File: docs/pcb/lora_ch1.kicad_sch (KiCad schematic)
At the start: 22 parts, among them J2 TYPE-C-31-M-12, J3 JST_2mm_LiPo, U1 ESP32-C3_SUPERMINI_TH, U2 TP4056-42-ESOP8, U3 DRV2605LDGS, U4 AP2112K-3.3

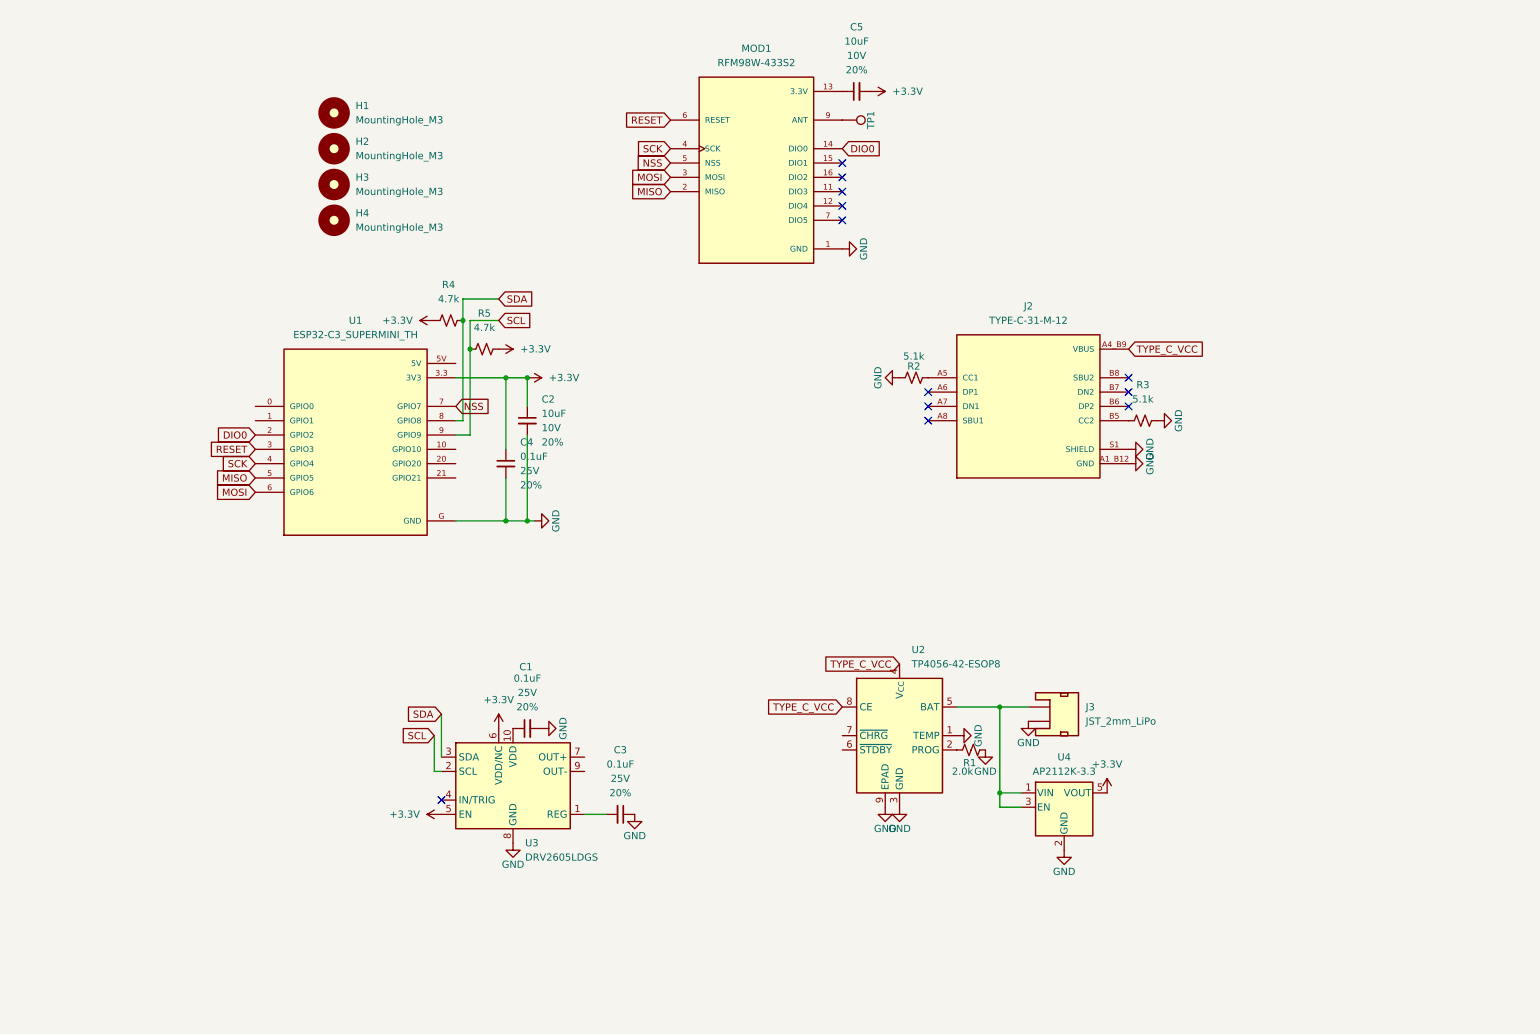
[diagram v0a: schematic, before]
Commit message: PCB schematic finished.
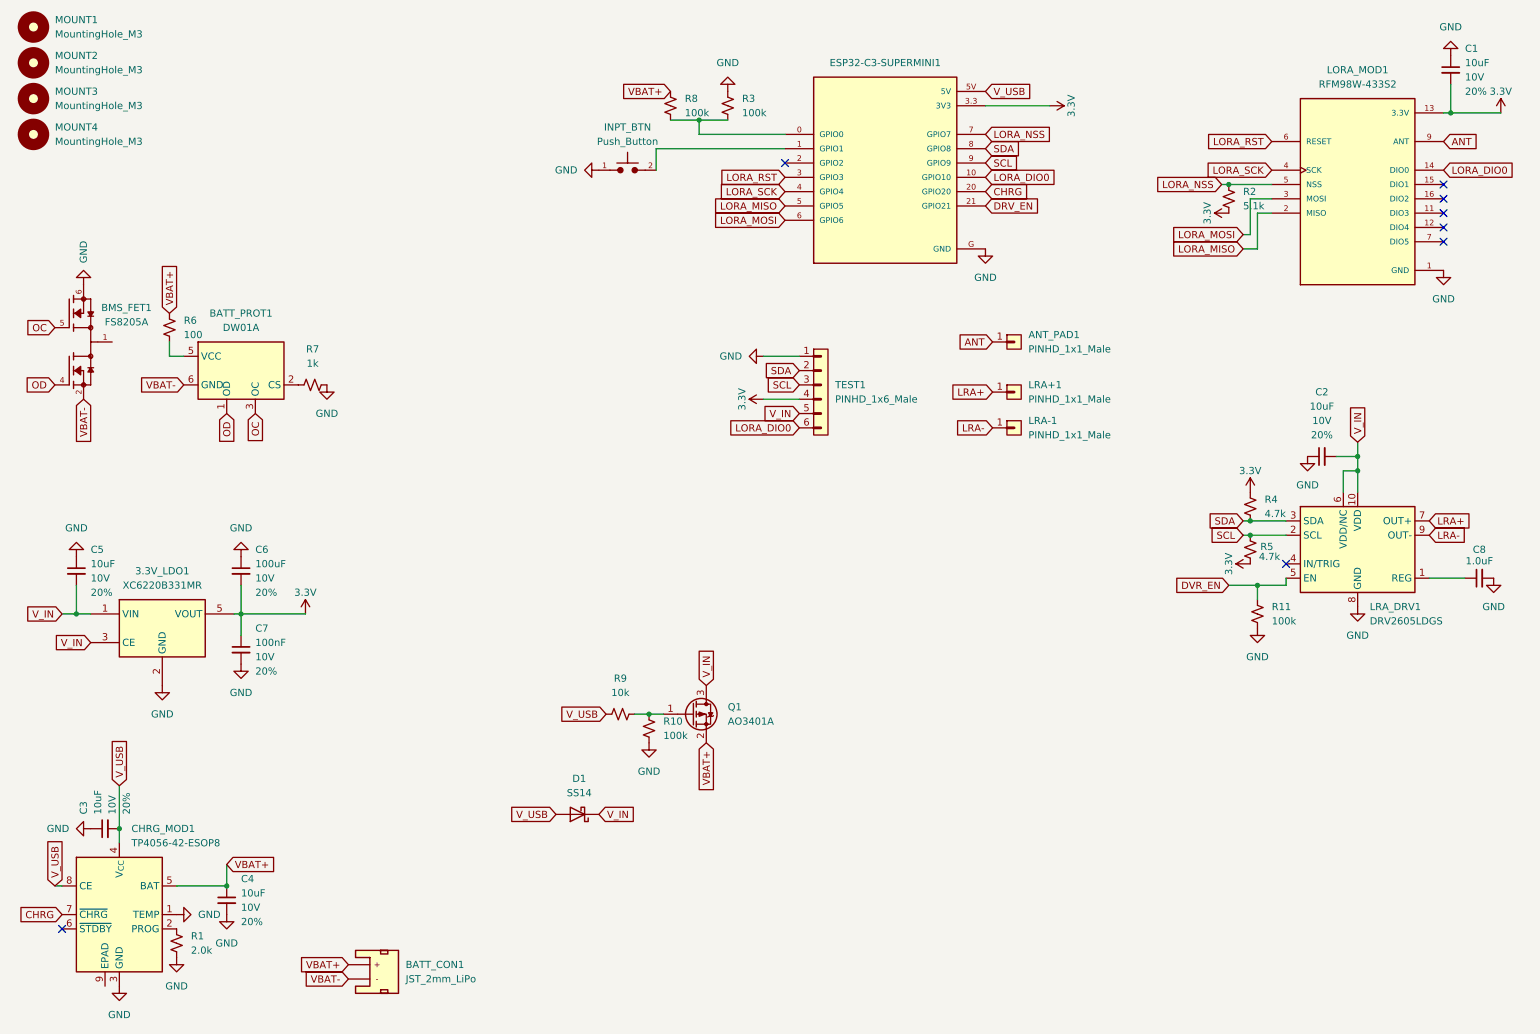
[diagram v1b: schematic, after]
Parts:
- removed C1, C3, C4: 0.1uF, PCM_SparkFun-Capacitor:C_0603_1608Metric, symbol PCM_SparkFun-Capacitor:0.1uF_0603_25V_20%
- removed J2: TYPE-C-31-M-12, TYPE-C-31-M-12:HRO_TYPE-C-31-M-12, symbol TYPE-C-31-M-12:TYPE-C-31-M-12
- removed J3: JST_2mm_LiPo, PCM_SparkFun-Connector:JST_1x02_P2.0mm_Horizontal_SMD, symbol PCM_SparkFun-Connector:Conn_01x02_JST_P2.0mm_Horizontal_SMD
- removed R3: 5.1k, PCM_SparkFun-Resistor:R_0603_1608Metric, symbol PCM_SparkFun-Resistor:5.1k_0603
- removed TP1: 1.25mm, PCM_SparkFun-Connector:TestPoint-1.25mm, symbol PCM_SparkFun-Connector:TestPoint_1.25mm
- removed U2: TP4056-42-ESOP8, Package_SO:SOIC-8-1EP_3.9x4.9mm_P1.27mm_EP2.41x3.3mm_ThermalVias, symbol Battery_Management:TP4056-42-ESOP8
- removed U3: DRV2605LDGS, Package_SO:VSSOP-10_3x3mm_P0.5mm, symbol Driver_Haptic:DRV2605LDGS
- removed U4: AP2112K-3.3, Package_TO_SOT_SMD:SOT-23-5, symbol Regulator_Linear:AP2112K-3.3
- added 3.3V_LDO1: XC6220B331MR, Package_TO_SOT_SMD:SOT-23-5, symbol Regulator_Linear:XC6220B331MR
- added ANT_PAD1, LRA+1, LRA-1: PINHD_1x1_Male, Connector_Pin:Pin_D1.0mm_L10.0mm_LooseFit, symbol PCM_SL_Pin_Headers:PINHD_1x1_Male
- added BATT_CON1: JST_2mm_LiPo, PCM_SparkFun-Connector:JST_1x02_P2.0mm_Horizontal_SMD, symbol PCM_SparkFun-Connector:Conn_01x02_JST_P2.0mm_Horizontal_SMD_LiPo
- added BATT_PROT1: DW01A, Package_TO_SOT_SMD:SOT-23-6, symbol Battery_Management:DW01A
- added BMS_FET1: FS8205A, FS8205A:SOP65P640X120-8N, symbol FS8205A:FS8205A
- added C1, C3, C4: 10uF, PCM_SparkFun-Capacitor:C_0603_1608Metric, symbol PCM_SparkFun-Capacitor:10uF_0603_10V_20%
- added C6: 100uF, PCM_SparkFun-Capacitor:C_1206_3216Metric, symbol PCM_SparkFun-Capacitor:100uF_1206_50V_10%
- added C7: 100nF, PCM_SparkFun-Capacitor:C_0603_1608Metric, symbol PCM_SparkFun-Capacitor:100uF_1206_50V_10%
- added C8: 1.0uF, PCM_SparkFun-Capacitor:C_0603_1608Metric, symbol PCM_SparkFun-Capacitor:1.0uF_0603_16V_10%
- added CHRG_MOD1: TP4056-42-ESOP8, Package_SO:SOIC-8-1EP_3.9x4.9mm_P1.27mm_EP2.41x3.3mm_ThermalVias, symbol Battery_Management:TP4056-42-ESOP8
- added D1: SS14, Diode_SMD:D_SMA, symbol Diode:SS14
- added INPT_BTN: Push_Button, Button_Switch_THT:SW_PUSH_6mm, symbol PCM_SL_Devices:Push_Button
- added LRA_DRV1: DRV2605LDGS, Package_SO:VSSOP-10_3x3mm_P0.5mm, symbol Driver_Haptic:DRV2605LDGS
- added Q1: AO3401A, Package_TO_SOT_SMD:SOT-23, symbol Transistor_FET:AO3401A
- added R10, R11, R3, R8: 100k, PCM_SparkFun-Resistor:R_0603_1608Metric, symbol PCM_SparkFun-Resistor:100k_0603
- added R6: 100, PCM_SparkFun-Resistor:R_0603_1608Metric, symbol PCM_SparkFun-Resistor:100_0603
- added R7: 1k, PCM_SparkFun-Resistor:R_0603_1608Metric, symbol PCM_SparkFun-Resistor:1k_0603
- added R9: 10k, PCM_SparkFun-Resistor:R_0603_1608Metric, symbol PCM_SparkFun-Resistor:10k_0603
- added TEST1: PINHD_1x6_Male, Connector_PinHeader_2.54mm:PinHeader_1x06_P2.54mm_Vertical, symbol PCM_SL_Pin_Headers:PINHD_1x6_Male
- C2, C5: LCSC (none) -> C19702
- R1: LCSC (none) -> C22975
- R4, R5: LCSC (none) -> C23162
- renumbered U1 to ESP32-C3-SUPERMINI1, MOD1 to LORA_MOD1, H1 to MOUNT1, H2 to MOUNT2, H3 to MOUNT3, H4 to MOUNT4
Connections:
- net NSS is gone; now on net LORA_NSS: ESP32-C3-SUPERMINI1.7 (GPIO7), LORA_MOD1.5 (NSS), LORA_MOD1.5_1 (NSS)
- net 3.3V: now also ESP32-C3-SUPERMINI1.3.3 (3V3), R2.1, R4.2, R5.1, 3.3V_LDO1.5 (VOUT), C1.2, C6.2, C7.1, TEST1.4; no longer C5.1
- net GND: now also C2.1, C5.1, R1.1, 3.3V_LDO1.2 (GND), BMS_FET1.6, BMS_FET1.7, C1.1, C3.1, C4.2, C6.1, C7.2, C8.2, CHRG_MOD1.1 (TEMP), CHRG_MOD1.3 (GND), INPT_BTN.1, LRA_DRV1.8 (GND), R10.1, R11.1, R3.2, R7.2, TEST1.1; no longer C2.2, R1.2, R2.1
- net SCL: now also R5.2, LRA_DRV1.2 (SCL), TEST1.3; no longer R5.1
- net SDA: now also R4.1, LRA_DRV1.3 (SDA), TEST1.2; no longer R4.2
- net ANT: now reaches LORA_MOD1.9 (ANT), LORA_MOD1.9_1 (ANT)
- net ANT: now also ANT_PAD1.1
- net at ESP32-C3-SUPERMINI1.0 (GPIO0): now also R3.1, R8.1
- net at ESP32-C3-SUPERMINI1.1 (GPIO1): now also INPT_BTN.2
- net LORA_DIO0: now reaches ESP32-C3-SUPERMINI1.10 (GPIO10)
- net LORA_DIO0: now also LORA_MOD1.14 (DIO0), LORA_MOD1.14_1 (DIO0), TEST1.6
- net CHRG: now reaches ESP32-C3-SUPERMINI1.20 (GPIO20)
- net CHRG: now also CHRG_MOD1.7 (~{CHRG})
- net DRV_EN: now reaches ESP32-C3-SUPERMINI1.21 (GPIO21)
- net V_USB: now reaches ESP32-C3-SUPERMINI1.5V
- net V_USB: now also C3.2, CHRG_MOD1.4 (V_{CC}), CHRG_MOD1.8 (CE), D1.2 (A), R9.1
- net LORA_NSS: now reaches R2.2
- removed net +3.3V: C2.1, C5.2, ESP32-C3-SUPERMINI1.3.3 (3V3), R4.1, R5.2
- removed net DIO0: ESP32-C3-SUPERMINI1.2 (GPIO2), LORA_MOD1.14 (DIO0), LORA_MOD1.14_1 (DIO0)
- net MISO renamed LORA_MISO
- net MOSI renamed LORA_MOSI
- net RESET renamed LORA_RST
- net SCK renamed LORA_SCK
- new net: Q1.1 (G), R10.2, R9.2
- new net: BATT_PROT1.5 (VCC), R6.2
- new net: BATT_PROT1.2 (CS), R7.1
- new net: CHRG_MOD1.2 (PROG), R1.2
- new net: BMS_FET1.1, BMS_FET1.8
- new net: C8.1, LRA_DRV1.1 (REG)
- new net DVR_EN: LRA_DRV1.5 (EN), R11.2
- new net LRA+: LRA+1.1, LRA_DRV1.7 (OUT+)
- new net LRA-: LRA-1.1, LRA_DRV1.9 (OUT-)
- new net OC: BATT_PROT1.3 (OC), BMS_FET1.5
- new net OD: BATT_PROT1.1 (OD), BMS_FET1.4
- new net VBAT+: BATT_CON1.2 (+), C4.1, CHRG_MOD1.5 (BAT), Q1.2 (S), R6.1, R8.2
- new net VBAT-: BATT_CON1.1 (-), BATT_PROT1.6 (GND), BMS_FET1.2, BMS_FET1.3
- new net V_IN: 3.3V_LDO1.1 (VIN), 3.3V_LDO1.3 (CE), C2.2, C5.2, D1.1 (K), LRA_DRV1.10 (VDD), LRA_DRV1.6 (VDD/NC), Q1.3 (D), TEST1.5
- no-connect marks 12 -> 8
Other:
- moved on the sheet: ESP32-C3-SUPERMINI1, LORA_MOD1, MOUNT1, MOUNT2, MOUNT3, MOUNT4
